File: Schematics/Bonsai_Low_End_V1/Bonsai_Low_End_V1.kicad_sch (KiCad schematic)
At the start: 6 parts, among them U1 MOUDLE-SEEEDUINO-XIAO-ESP32C3, U2 MAX30101EFD

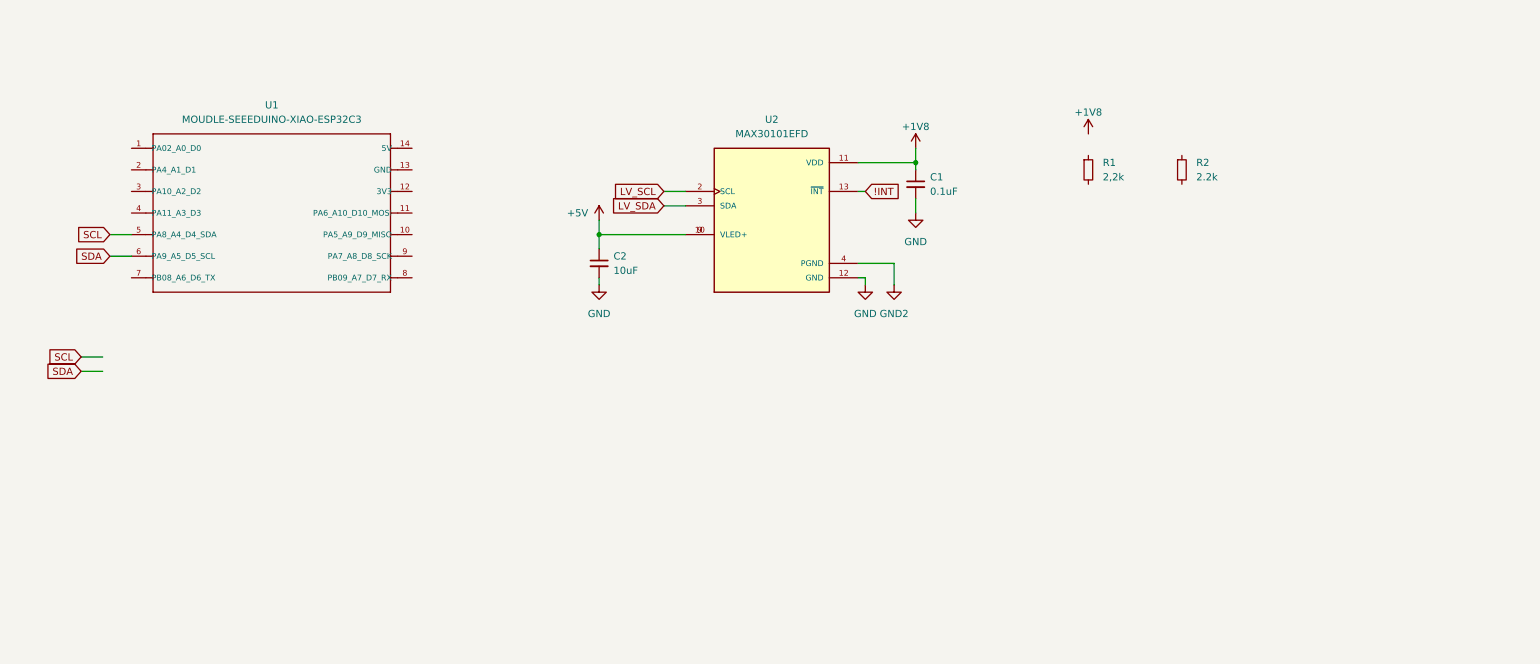
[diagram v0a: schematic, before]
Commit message: Before Everything Breaks
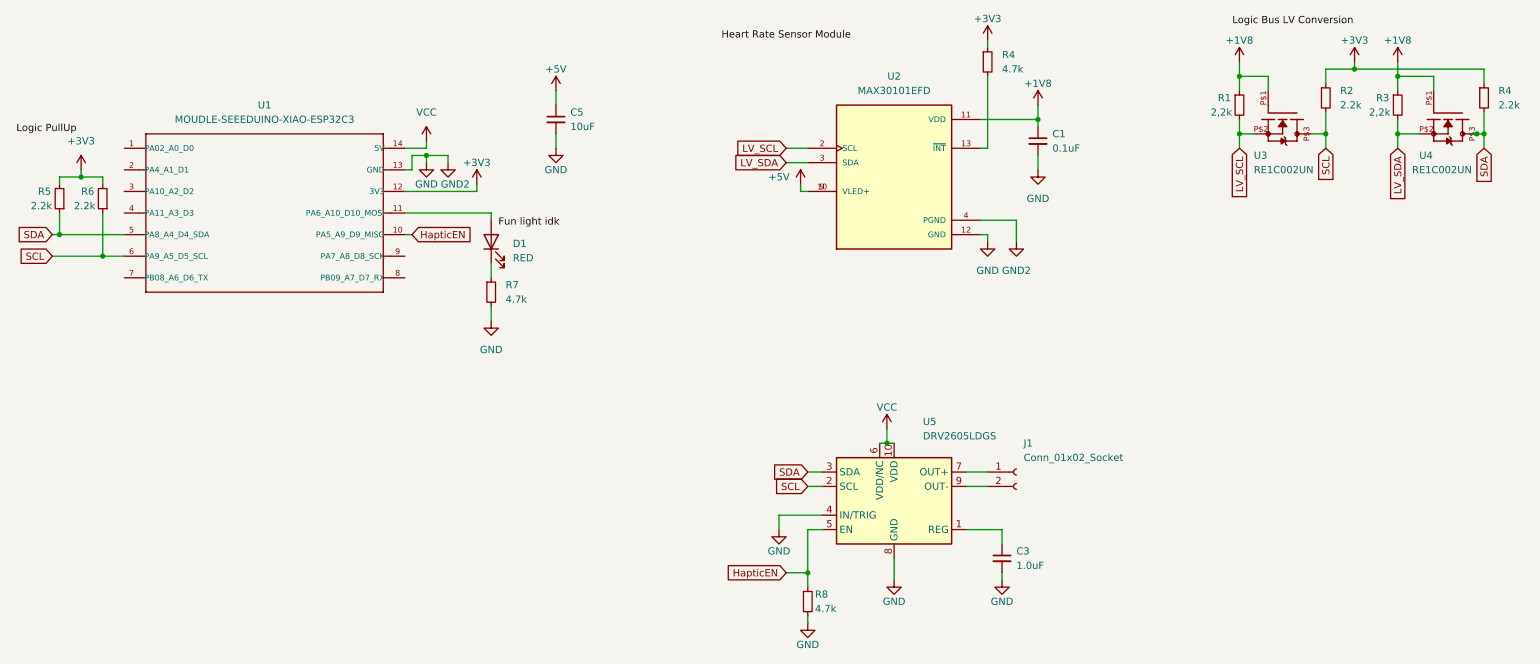
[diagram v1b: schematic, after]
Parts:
- removed C2: 10uF, symbol Device:C_Small
- added C3: 1.0uF, symbol Device:C_Small
- added C5: 10uF, symbol Device:C_Small
- added D1: RED, symbol Device:LED
- added J1: Conn_01x02_Socket, symbol Connector:Conn_01x02_Socket
- added R3: 2,2k, symbol Device:R_Small
- added R4, R7, R8: 4.7k, symbol Device:R_Small
- added R4, R5, R6: 2.2k, symbol Device:R_Small
- added U3, U4: RE1C002UN, RE1C002UN:EMT3F, symbol RE1C002UN:RE1C002UN
- added U5: DRV2605LDGS, Package_SO:VSSOP-10_3x3mm_P0.5mm, symbol Driver_Haptic:DRV2605LDGS
- U1: footprint MOUDLE14P-SMD-2.54-21X17.8MM -> xiao ESP32C3_PCB:MOUDLE14P-SMD-2.54-21X17.8MM
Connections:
- net GND2 is gone; now on net GND: U2.4 (PGND)
- net +1V8: now also R1.1, R3.1, U3.P$1, U4.P$1
- net +5V: now also C5.1
- net GND: now also U1.13 (GND), C3.2, C5.2, R7.2, R8.2, U5.4 (IN/TRIG), U5.8 (GND)
- net LV_SCL: now also R1.2, U3.P$2
- net LV_SDA: now also R3.2, U4.P$2
- net SCL: now also R2.2, U1.6 (PA9_A5_D5_SCL), R6.1, U3.P$3, U5.2 (SCL); no longer U1.5 (PA8_A4_D4_SDA)
- net SDA: now also U1.5 (PA8_A4_D4_SDA), R4.2, R5.1, U4.P$3, U5.3 (SDA); no longer U1.6 (PA9_A5_D5_SCL)
- net +3V3: now reaches R2.1
- net +3V3: now also U1.12 (3V3), R4.1, R4.1, R5.2, R6.2
- net HapticEN: now reaches U1.10 (PA5_A9_D9_MISO)
- net HapticEN: now also R8.1, U5.5 (EN)
- net at U1.11 (PA6_A10_D10_MOSI): now also D1.2 (A)
- net VCC: now reaches U1.14 (5V)
- net VCC: now also U5.10 (VDD), U5.6 (VDD/NC)
- net !INT: no longer names the net of U2.13 (~{INT})
- net !INT: now also R4.2
- new net: D1.1 (K), R7.1
- new net: C3.1, U5.1 (REG)
- new net: J1.1 (Pin_1), U5.7 (OUT+)
- new net: J1.2 (Pin_2), U5.9 (OUT-)
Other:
- moved on the sheet: C1, R1, R2, U1, U2
